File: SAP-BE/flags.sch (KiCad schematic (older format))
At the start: 3 parts, among them U48 74LS173

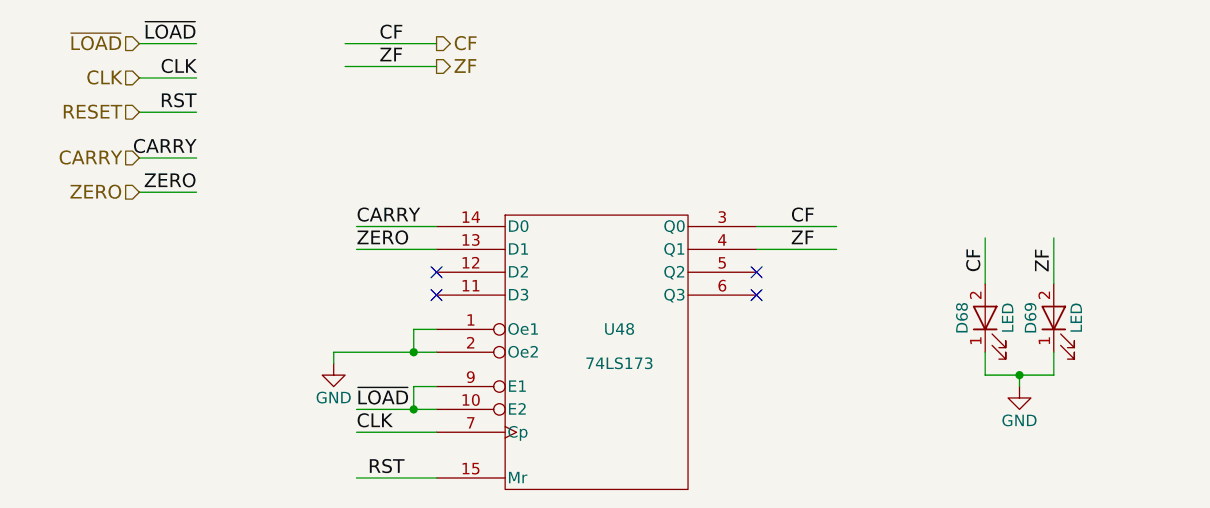
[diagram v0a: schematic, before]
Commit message: fixup flags schematic settings
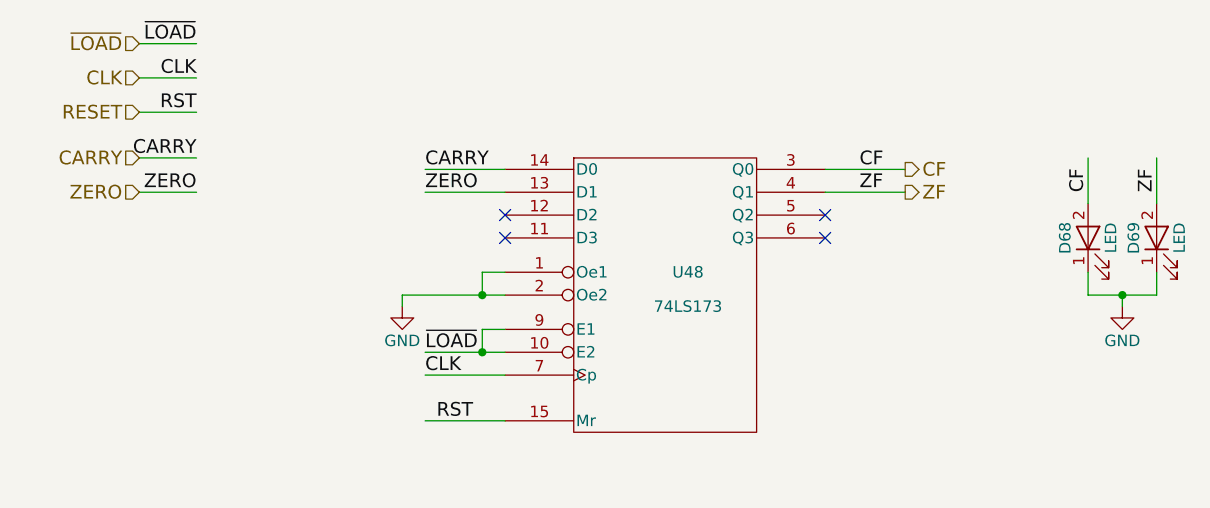
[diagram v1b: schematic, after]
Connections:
- wire segments 26 -> 27
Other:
- moved on the sheet: D68, D69, U48
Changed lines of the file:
@@
 encoding utf-8
 Sheet 12 12
-Title ""
-Date ""
-Rev ""
-Comp ""
-Comment1 ""
-Comment2 ""
+Title "Simple As Possible computer by Ben Eater"
+Date "2017-05-10"
+Rev "1"
+Comp "Schematic released as CC BY-SA"
+Comment1 "Schematic capture by Vincent Sanders"
+Comment2 "Flags register"
 Comment3 ""
 Comment4 ""
@@
 Text HLabel 1300 1600 0    60   Input ~ 0
 ZERO
-Text HLabel 2600 950  2    60   Output ~ 0
+Text HLabel 4650 1500 2    60   Output ~ 0
 CF
-Text HLabel 2600 1050 2    60   Output ~ 0
+Text HLabel 4650 1600 2    60   Output ~ 0
 ZF
 $Comp
 L 74LS173 U48
 U 1 1 5AD47646
-P 3300 2300
-F 0 "U48" H 3400 2400 50  0000 C CNN
-F 1 "74LS173" H 3400 2250 50  0000 C CNN
-F 2 "" H 3300 2300 50  0000 C CNN
-F 3 "" H 3300 2300 50  0000 C CNN
-	1    3300 2300
+P 3600 2050
+F 0 "U48" H 3700 2150 50  0000 C CNN
+F 1 "74LS173" H 3700 2000 50  0000 C CNN
+F 2 "" H 3600 2050 50  0000 C CNN
+F 3 "" H 3600 2050 50  0000 C CNN
+	1    3600 2050
 	1    0    0    -1
 $EndComp
 Text Label 1550 950  2    60   ~ 0
 ~LOAD
-Text Label 2250 2550 0    60   ~ 0
+Text Label 2550 2300 0    60   ~ 0
 ~LOAD
 $Comp
 L GND #PWR090
 U 1 1 5AD4767C
-P 2150 2350
-F 0 "#PWR090" H 2150 2100 50  0001 C CNN
-F 1 "GND" H 2150 2200 50  0000 C CNN
-F 2 "" H 2150 2350 50  0000 C CNN
-F 3 "" H 2150 2350 50  0000 C CNN
-	1    2150 2350
+P 2450 2100
+F 0 "#PWR090" H 2450 1850 50  0001 C CNN
+F 1 "GND" H 2450 1950 50  0000 C CNN
+F 2 "" H 2450 2100 50  0000 C CNN
+F 3 "" H 2450 2100 50  0000 C CNN
+	1    2450 2100
 	1    0    0    -1
 $EndComp
-Text Label 2250 1750 0    60   ~ 0
+Text Label 2550 1500 0    60   ~ 0
 CARRY
-Text Label 2250 1850 0    60   ~ 0
+Text Label 2550 1600 0    60   ~ 0
 ZERO
 Text Label 1550 1450 2    60   ~ 0
@@
 Text Label 1550 1250 2    60   ~ 0
 RST
-Text Label 2300 2850 0    60   ~ 0
+Text Label 2600 2600 0    60   ~ 0
 RST
 Wire Wire Line
 	1550 950  1300 950
 Wire Wire Line
-	2250 2550 2600 2550
+	2550 2300 2800 2300
 Wire Wire Line
-	2500 2550 2500 2450
+	2800 2300 2900 2300
 Wire Wire Line
-	2500 2450 2600 2450
-Connection ~ 2500 2550
+	2800 2300 2800 2200
 Wire Wire Line
-	2600 2300 2150 2300
+	2800 2200 2900 2200
+Connection ~ 2800 2300
 Wire Wire Line
-	2150 2300 2150 2350
+	2900 2050 2800 2050
 Wire Wire Line
-	2600 2200 2500 2200
+	2800 2050 2450 2050
 Wire Wire Line
-	2500 2200 2500 2300
-Connection ~ 2500 2300
+	2450 2050 2450 2100
 Wire Wire Line
-	2250 1750 2600 1750
+	2900 1950 2800 1950
 Wire Wire Line
-	2250 1850 2600 1850
+	2800 1950 2800 2050
+Connection ~ 2800 2050
+Wire Wire Line
+	2550 1500 2900 1500
+Wire Wire Line
+	2550 1600 2900 1600
 Wire Wire Line
 	1550 1450 1300 1450
@@
 	1550 1600 1300 1600
 Wire Wire Line
-	4350 1850 4000 1850
+	4650 1600 4300 1600
 Wire Wire Line
-	4350 1750 4000 1750
+	4650 1500 4300 1500
 Wire Wire Line
 	1550 1250 1300 1250
@@
 	1550 1100 1300 1100
 Wire Wire Line
-	2250 2850 2600 2850
+	2550 2600 2900 2600
 Wire Wire Line
-	2250 2650 2600 2650
-Text Label 2250 2650 0    60   ~ 0
+	2550 2400 2900 2400
+Text Label 2550 2400 0    60   ~ 0
 CLK
-Wire Wire Line
-	2200 950  2600 950
-Wire Wire Line
-	2200 1050 2600 1050
-Text Label 2350 950  0    60   ~ 0
+Text Label 4450 1500 0    60   ~ 0
 CF
-Text Label 2350 1050 0    60   ~ 0
+Text Label 4450 1600 0    60   ~ 0
 ZF
-Text Label 4150 1750 0    60   ~ 0
-CF
-Text Label 4150 1850 0    60   ~ 0
-ZF
-NoConn ~ 4000 1950
-NoConn ~ 4000 2050
-NoConn ~ 2600 1950
-NoConn ~ 2600 2050
+NoConn ~ 4300 1700
+NoConn ~ 4300 1800
+NoConn ~ 2900 1700
+NoConn ~ 2900 1800
 $Comp
 L LED D68
 U 1 1 5AD4AD3C
-P 5000 2150
-F 0 "D68" H 5000 2250 50  0000 C CNN
-F 1 "LED" H 5000 2050 50  0000 C CNN
-F 2 "" H 5000 2150 50  0000 C CNN
-F 3 "" H 5000 2150 50  0000 C CNN
-	1    5000 2150
+P 5450 1800
+F 0 "D68" H 5450 1900 50  0000 C CNN
+F 1 "LED" H 5450 1700 50  0000 C CNN
+F 2 "" H 5450 1800 50  0000 C CNN
+F 3 "" H 5450 1800 50  0000 C CNN
+	1    5450 1800
 	0    -1   -1   0
 $EndComp
@@
 L LED D69
 U 1 1 5AD4AD4E
-P 5300 2150
-F 0 "D69" H 5300 2250 50  0000 C CNN
-F 1 "LED" H 5300 2050 50  0000 C CNN
-F 2 "" H 5300 2150 50  0000 C CNN
-F 3 "" H 5300 2150 50  0000 C CNN
-	1    5300 2150
+P 5750 1800
+F 0 "D69" H 5750 1900 50  0000 C CNN
+F 1 "LED" H 5750 1700 50  0000 C CNN
+F 2 "" H 5750 1800 50  0000 C CNN
+F 3 "" H 5750 1800 50  0000 C CNN
+	1    5750 1800
 	0    -1   -1   0
 $EndComp
@@
 L GND #PWR091
 U 1 1 5AD4AD59
-P 5150 2450
-F 0 "#PWR091" H 5150 2200 50  0001 C CNN
-F 1 "GND" H 5150 2300 50  0000 C CNN
-F 2 "" H 5150 2450 50  0000 C CNN
-F 3 "" H 5150 2450 50  0000 C CNN
-	1    5150 2450
+P 5600 2100
+F 0 "#PWR091" H 5600 1850 50  0001 C CNN
+F 1 "GND" H 5600 1950 50  0000 C CNN
+F 2 "" H 5600 2100 50  0000 C CNN
+F 3 "" H 5600 2100 50  0000 C CNN
+	1    5600 2100
 	1    0    0    -1
 $EndComp
 Wire Wire Line
-	5150 2450 5150 2400
+	5600 2100 5600 2050
 Wire Wire Line
-	5000 2400 5300 2400
+	5450 2050 5600 2050
 Wire Wire Line
-	5000 2400 5000 2300
+	5600 2050 5750 2050
 Wire Wire Line
-	5300 2400 5300 2300
-Connection ~ 5150 2400
+	5450 2050 5450 1950
 Wire Wire Line
-	5000 1800 5000 2000
+	5750 2050 5750 1950
+Connection ~ 5600 2050
 Wire Wire Line
-	5300 1800 5300 2000
-Text Label 5000 1950 1    60   ~ 0
+	5450 1450 5450 1650
+Wire Wire Line
+	5750 1450 5750 1650
+Text Label 5450 1600 1    60   ~ 0
 CF
-Text Label 5300 1950 1    60   ~ 0
+Text Label 5750 1600 1    60   ~ 0
 ZF
 $EndSCHEMATC
